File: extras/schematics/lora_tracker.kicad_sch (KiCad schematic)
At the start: 27 parts, among them J1 ANT, J4 Conn_01x03_Female, SW1 SW_Push, U1 ESP32, U2 E22-400M30S, U3 RA-01, U4 INP441, U5 MAX98357A, U6 SSD1306, U7 EC11

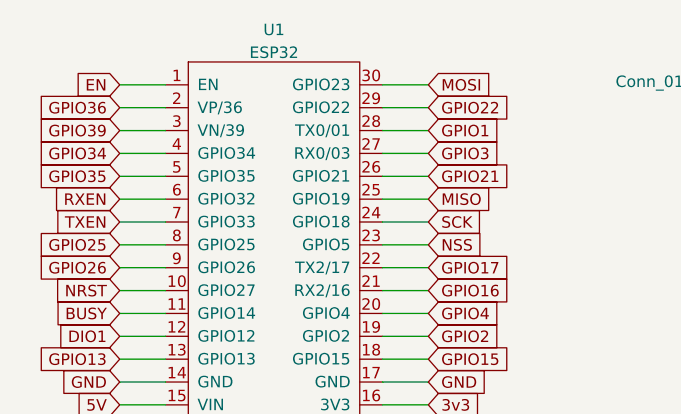
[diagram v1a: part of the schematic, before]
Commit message: Update schematics
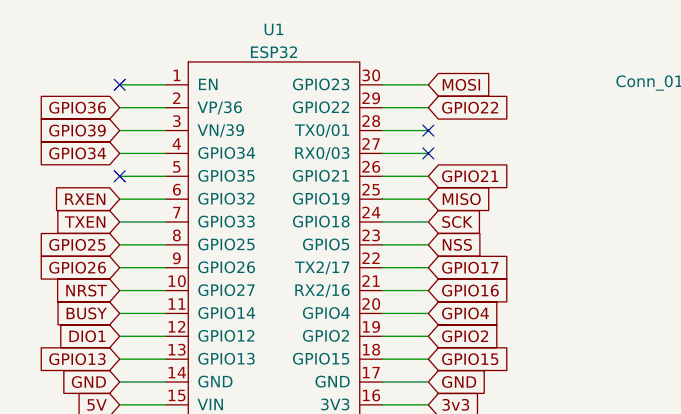
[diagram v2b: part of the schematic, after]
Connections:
- net EN: no longer names the net of U1.1 (EN)
- net GPIO1: no longer names the net of U1.28 (TX0/01)
- net GPIO3: no longer names the net of U1.27 (RX0/03)
- net GPIO35: no longer names the net of U1.5 (GPIO35)
- no-connect marks 5 -> 9
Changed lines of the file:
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@@
   )
   (no_connect (at 205.74 71.12))
+  (no_connect (at 60.96 29.21))
   (no_connect (at 175.26 54.61))
+  (no_connect (at 60.96 26.67))
+  (no_connect (at 26.67 31.75))
+  (no_connect (at 26.67 21.59))
   (no_connect (at 175.26 52.07))
   (no_connect (at 175.26 49.53))
@@
     )
   )
+  (global_label "GPIO21" (shape input) (at 60.96 31.75 0) (fields_autoplaced)
+    (effects (font (size 1.27 1.27)) (justify left))
+    (property "Intersheet References" "${INTERSHEET_REFS}" (id 0) (at 70.1785 31.6706 0)
+      (effects (font (size 1.27 1.27)) (justify left) hide)
+    )
+  )
   (global_label "DIO1" (shape input) (at 259.08 81.28 0) (fields_autoplaced)
     (effects (font (size 1.27 1.27)) (justify left))
@@
     (property "Intersheet References" "${INTERSHEET_REFS}" (id 0) (at 118.11 182.88 0)
       (effects (font (size 1.27 1.27)) hide)
+    )
+  )
+  (global_label "GPIO2" (shape input) (at 60.96 49.53 0) (fields_autoplaced)
+    (effects (font (size 1.27 1.27)) (justify left))
+    (property "Intersheet References" "${INTERSHEET_REFS}" (id 0) (at 68.969 49.4506 0)
+      (effects (font (size 1.27 1.27)) (justify left) hide)
     )
   )
@@
     )
   )
-  (global_label "EN" (shape input) (at 26.67 21.59 180) (fields_autoplaced)
-    (effects (font (size 1.27 1.27)) (justify right))
-    (property "Intersheet References" "${INTERSHEET_REFS}" (id 0) (at -25.4 -30.48 0)
-      (effects (font (size 1.27 1.27)) hide)
-    )
-  )
   (global_label "GPIO16" (shape input) (at 74.93 167.64 180) (fields_autoplaced)
     (effects (font (size 1.27 1.27)) (justify right))
@@
     )
   )
-  (global_label "GPIO15" (shape input) (at 60.96 52.07 0) (fields_autoplaced)
-    (effects (font (size 1.27 1.27)) (justify left))
-    (property "Intersheet References" "${INTERSHEET_REFS}" (id 0) (at -25.4 -35.56 0)
-      (effects (font (size 1.27 1.27)) hide)
-    )
-  )
   (global_label "GND" (shape input) (at 124.46 43.18 270) (fields_autoplaced)
     (effects (font (size 1.27 1.27)) (justify right))
@@
     )
   )
+  (global_label "GPIO4" (shape input) (at 60.96 46.99 0) (fields_autoplaced)
+    (effects (font (size 1.27 1.27)) (justify left))
+    (property "Intersheet References" "${INTERSHEET_REFS}" (id 0) (at 68.969 46.9106 0)
+      (effects (font (size 1.27 1.27)) (justify left) hide)
+    )
+  )
   (global_label "MISO" (shape input) (at 259.08 66.04 0) (fields_autoplaced)
     (effects (font (size 1.27 1.27)) (justify left))
@@
     )
   )
-  (global_label "GPIO3" (shape input) (at 60.96 29.21 0) (fields_autoplaced)
-    (effects (font (size 1.27 1.27)) (justify left))
-    (property "Intersheet References" "${INTERSHEET_REFS}" (id 0) (at -25.4 -30.48 0)
-      (effects (font (size 1.27 1.27)) hide)
-    )
-  )
   (global_label "GND" (shape input) (at 143.51 113.03 270) (fields_autoplaced)
     (effects (font (size 1.27 1.27)) (justify right))
@@
     )
   )
-  (global_label "GPIO35" (shape input) (at 26.67 31.75 180) (fields_autoplaced)
-    (effects (font (size 1.27 1.27)) (justify right))
-    (property "Intersheet References" "${INTERSHEET_REFS}" (id 0) (at -25.4 -30.48 0)
-      (effects (font (size 1.27 1.27)) hide)
-    )
-  )
   (global_label "MOSI" (shape input) (at 60.96 21.59 0) (fields_autoplaced)
-    (effects (font (size 1.27 1.27)) (justify left))
-    (property "Intersheet References" "${INTERSHEET_REFS}" (id 0) (at -25.4 -30.48 0)
-      (effects (font (size 1.27 1.27)) hide)
-    )
-  )
-  (global_label "GPIO2" (shape input) (at 60.96 49.53 0) (fields_autoplaced)
-    (effects (font (size 1.27 1.27)) (justify left))
-    (property "Intersheet References" "${INTERSHEET_REFS}" (id 0) (at -25.4 -35.56 0)
-      (effects (font (size 1.27 1.27)) hide)
-    )
-  )
-  (global_label "GPIO1" (shape input) (at 60.96 26.67 0) (fields_autoplaced)
     (effects (font (size 1.27 1.27)) (justify left))
     (property "Intersheet References" "${INTERSHEET_REFS}" (id 0) (at -25.4 -30.48 0)
@@
     )
   )
-  (global_label "GPIO4" (shape input) (at 60.96 46.99 0) (fields_autoplaced)
-    (effects (font (size 1.27 1.27)) (justify left))
-    (property "Intersheet References" "${INTERSHEET_REFS}" (id 0) (at -25.4 -33.02 0)
-      (effects (font (size 1.27 1.27)) hide)
-    )
-  )
   (global_label "MISO" (shape input) (at 147.32 54.61 180) (fields_autoplaced)
     (effects (font (size 1.27 1.27)) (justify right))
@@
   (global_label "GND" (shape input) (at 102.87 27.94 0) (fields_autoplaced)
     (effects (font (size 1.27 1.27)) (justify left))
-    (property "Intersheet References" "${INTERSHEET_REFS}" (id 0) (at -104.14 -123.19 0)
-      (effects (font (size 1.27 1.27)) hide)
-    )
-  )
-  (global_label "GPIO21" (shape input) (at 60.96 31.75 0) (fields_autoplaced)
-    (effects (font (size 1.27 1.27)) (justify left))
-    (property "Intersheet References" "${INTERSHEET_REFS}" (id 0) (at -25.4 -30.48 0)
-      (effects (font (size 1.27 1.27)) hide)
+    (property "Intersheet References" "${INTERSHEET_REFS}" (id 0) (at 109.0647 27.8606 0)
+      (effects (font (size 1.27 1.27)) (justify left) hide)
     )
   )
@@
     )
   )
+  (global_label "GPIO15" (shape input) (at 60.96 52.07 0) (fields_autoplaced)
+    (effects (font (size 1.27 1.27)) (justify left))
+    (property "Intersheet References" "${INTERSHEET_REFS}" (id 0) (at 70.1785 51.9906 0)
+      (effects (font (size 1.27 1.27)) (justify left) hide)
+    )
+  )
